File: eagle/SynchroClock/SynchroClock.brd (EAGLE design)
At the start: 84.8 x 45.7 mm, 37 parts, among them IC1 DS3231/SO, J1 VIN, U1 MCP1825-33, U2 ATTINY85-P

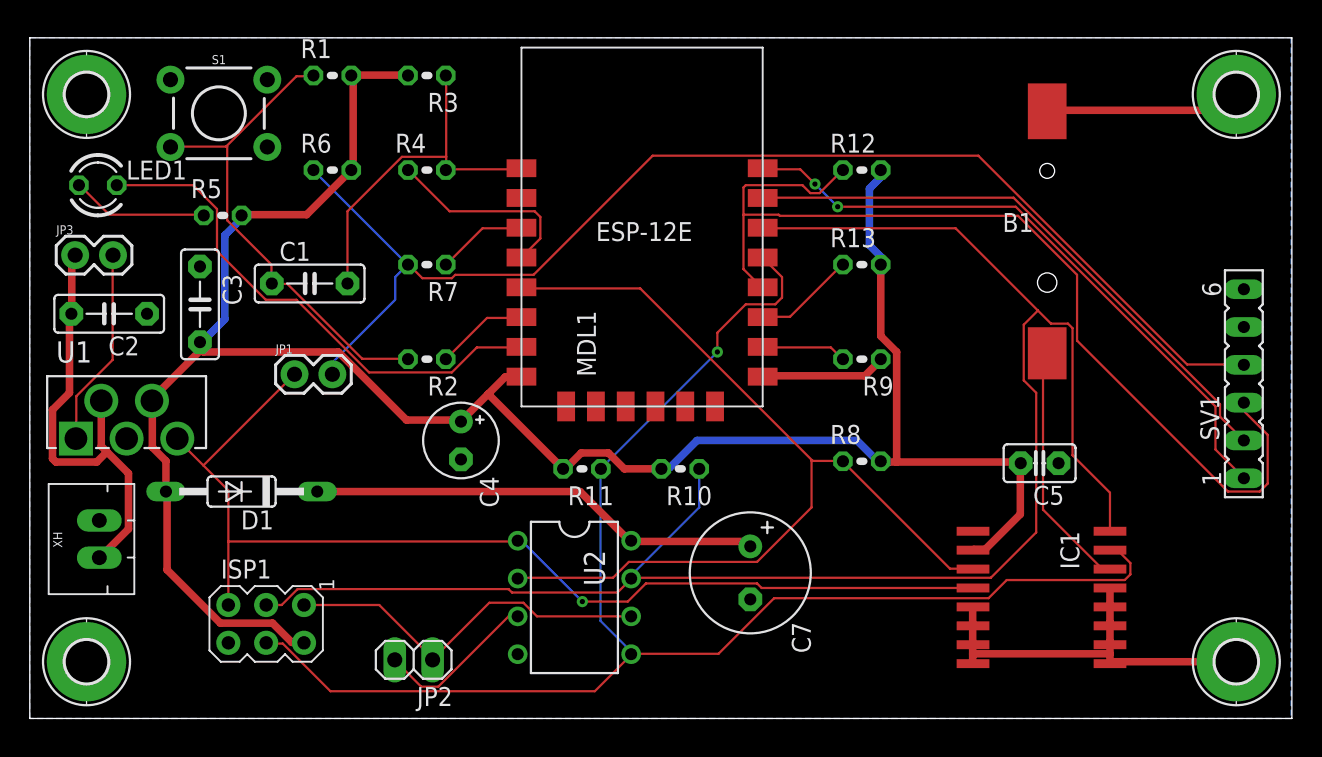
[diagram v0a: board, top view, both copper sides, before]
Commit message: board version 2.1
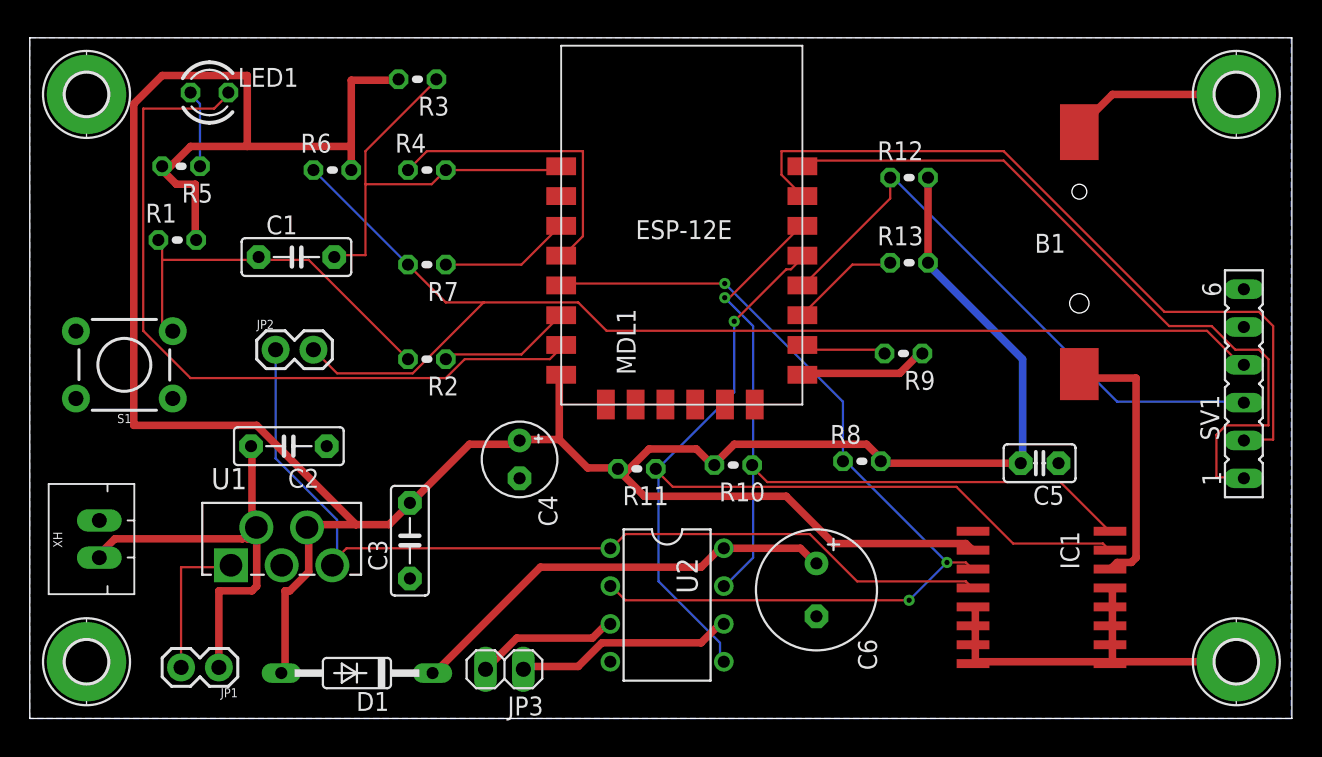
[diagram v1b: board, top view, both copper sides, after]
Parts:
- removed C7: 510uf, rcl:E3,5-8
- removed ISP1: AVRISP-6, SynchroClock:AVRISP
- added C6: 510uf, rcl:E3,5-8
- JP1: value PWRGD -> !SHDN
- JP2: value CLOCK -> PWRGD; device pinhead:1X02 -> SynchroClock:1X02
- JP3: value !SHDN -> CLOCK; device SynchroClock:1X02 -> pinhead:1X02
- moved JP3 40.1 mm to (31.9, 3.30), turned to 180 degrees
- moved JP2 22.8 mm to (16.5, 24.8), turned to 0 degrees
- moved C3 21.2 mm to (25.5, 11.9), turned to 90 degrees
- moved JP1 20.3 mm to (12.7, 3.43), turned to 180 degrees
- moved S1 18.0 mm to (6.35, 23.7), turned to 180 degrees
- moved R1 15.2 mm to (9.91, 32.1)
- moved C2 15.0 mm to (17.4, 18.3)
- moved D1 14.4 mm to (22.0, 3.05)
- moved U1 13.4 mm to (20.3, 13.8)
- moved LED1 9.74 mm to (12.1, 42.0)
- moved U2 6.24 mm to (42.8, 7.62)
- moved R5 4.33 mm to (10.2, 37.1), turned to 180 degrees
- moved C4 4.14 mm to (32.9, 17.4)
- moved R11 3.68 mm to (40.8, 16.8)
- moved R10 3.57 mm to (47.2, 17.0)
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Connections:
- net !SHDN: now also JP1.2; no longer JP3.2
- net +3V3: no longer ISP1.2
- net +5V: now also JP1.1; no longer JP3.1
- net A: now also JP3.1; no longer ISP1.1, JP2.1
- net ATVCC: now also C6.+; no longer C7.+
- net B: now also JP3.2; no longer JP2.2
- net GND: now also C6.-; no longer C7.-, ISP1.6
- net PWRGD: now also JP2.1; no longer ISP1.5, JP1.1
- net RST: now also JP2.2; no longer JP1.2
- net SCL: no longer ISP1.3
- net SDA: no longer ISP1.4
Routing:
- net SCL: track 117.2 -> 54.2 mm, vias 0 -> 1
- net +3V3: track 150.7 -> 198.7 mm
- net SDA: track 99.4 -> 66.4 mm
- net GPIO0: track 66.7 -> 40.0 mm
- net LED: track 34.8 -> 51.5 mm
- net PWRGD: track 73.7 -> 61.8 mm, vias 1 -> 0
- net RXD: track 39.6 -> 51.1 mm
- net A: track 25.5 -> 14.7 mm
- net TXD: track 42.7 -> 49.9 mm, vias 2 -> 0
- net N$1: track 33.4 -> 26.5 mm
- net GPIO16: track 13.4 -> 20.0 mm
- net REST: track 24.5 -> 29.6 mm
- net N$6: track 9.23 -> 5.22 mm
- net !SHDN: track 13.4 -> 10.1 mm
- net CH_PD: track 6.11 -> 8.81 mm
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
